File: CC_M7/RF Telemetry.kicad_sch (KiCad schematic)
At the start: 24 parts, among them U6 nRF52820-QDxx, U7 NRF21540-QDAA-R7, Y2 32MHz

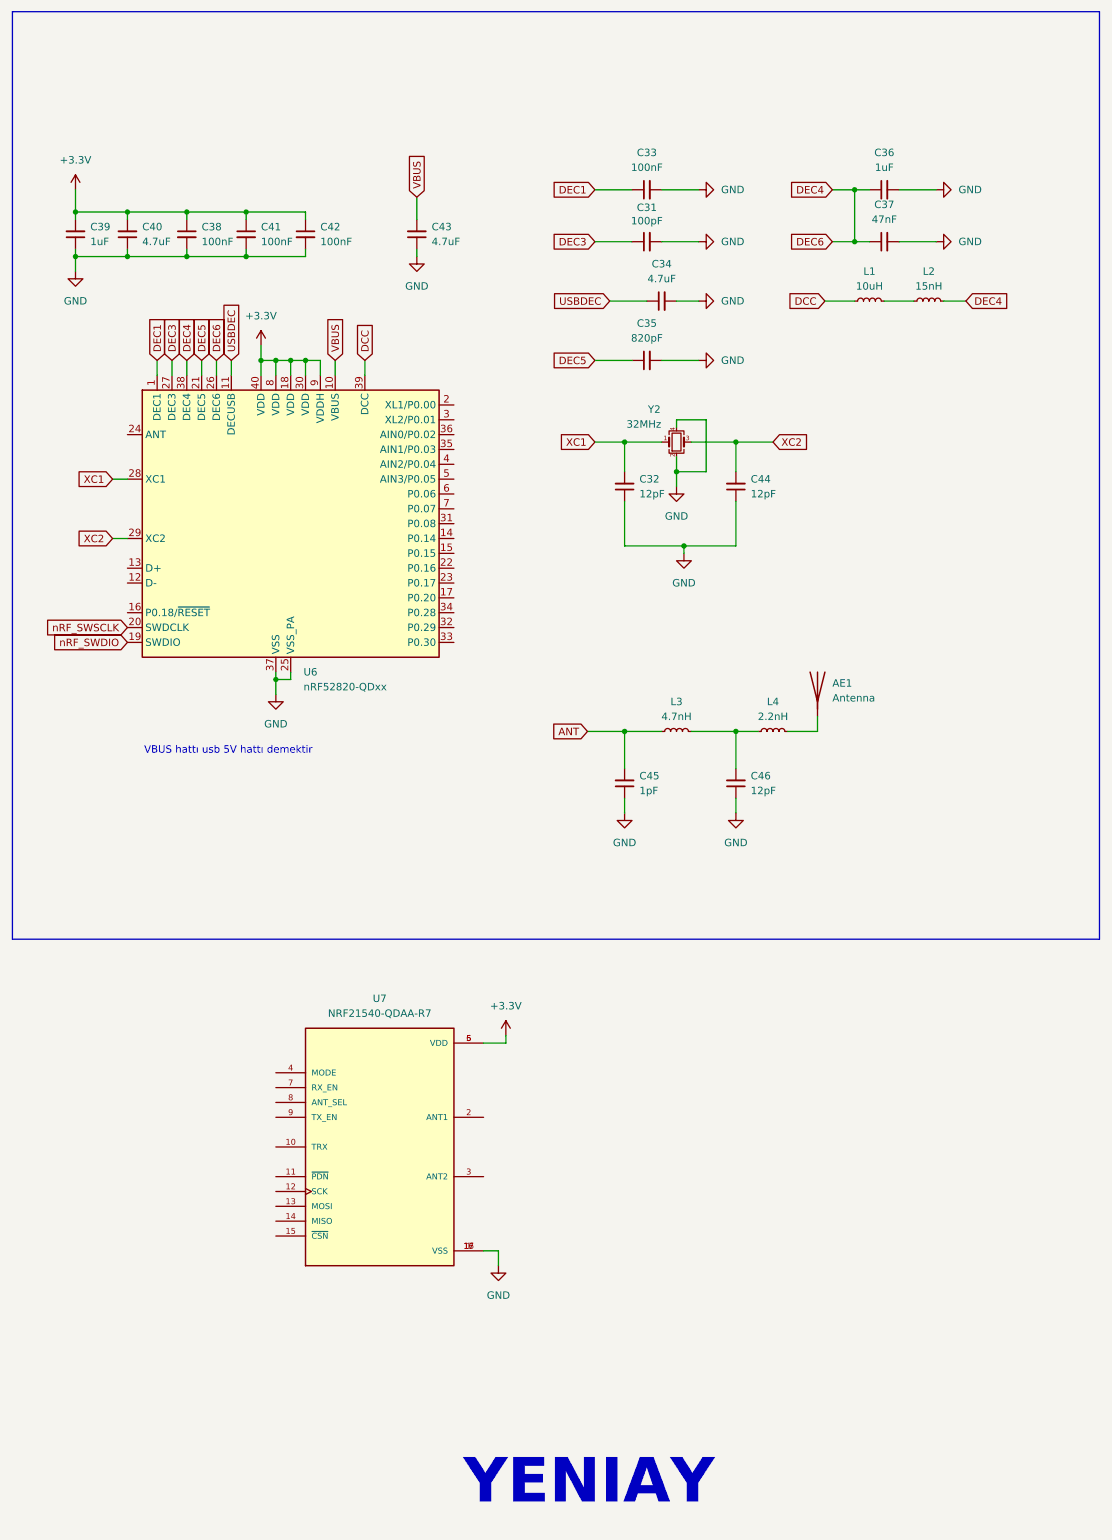
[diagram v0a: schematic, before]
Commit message: update
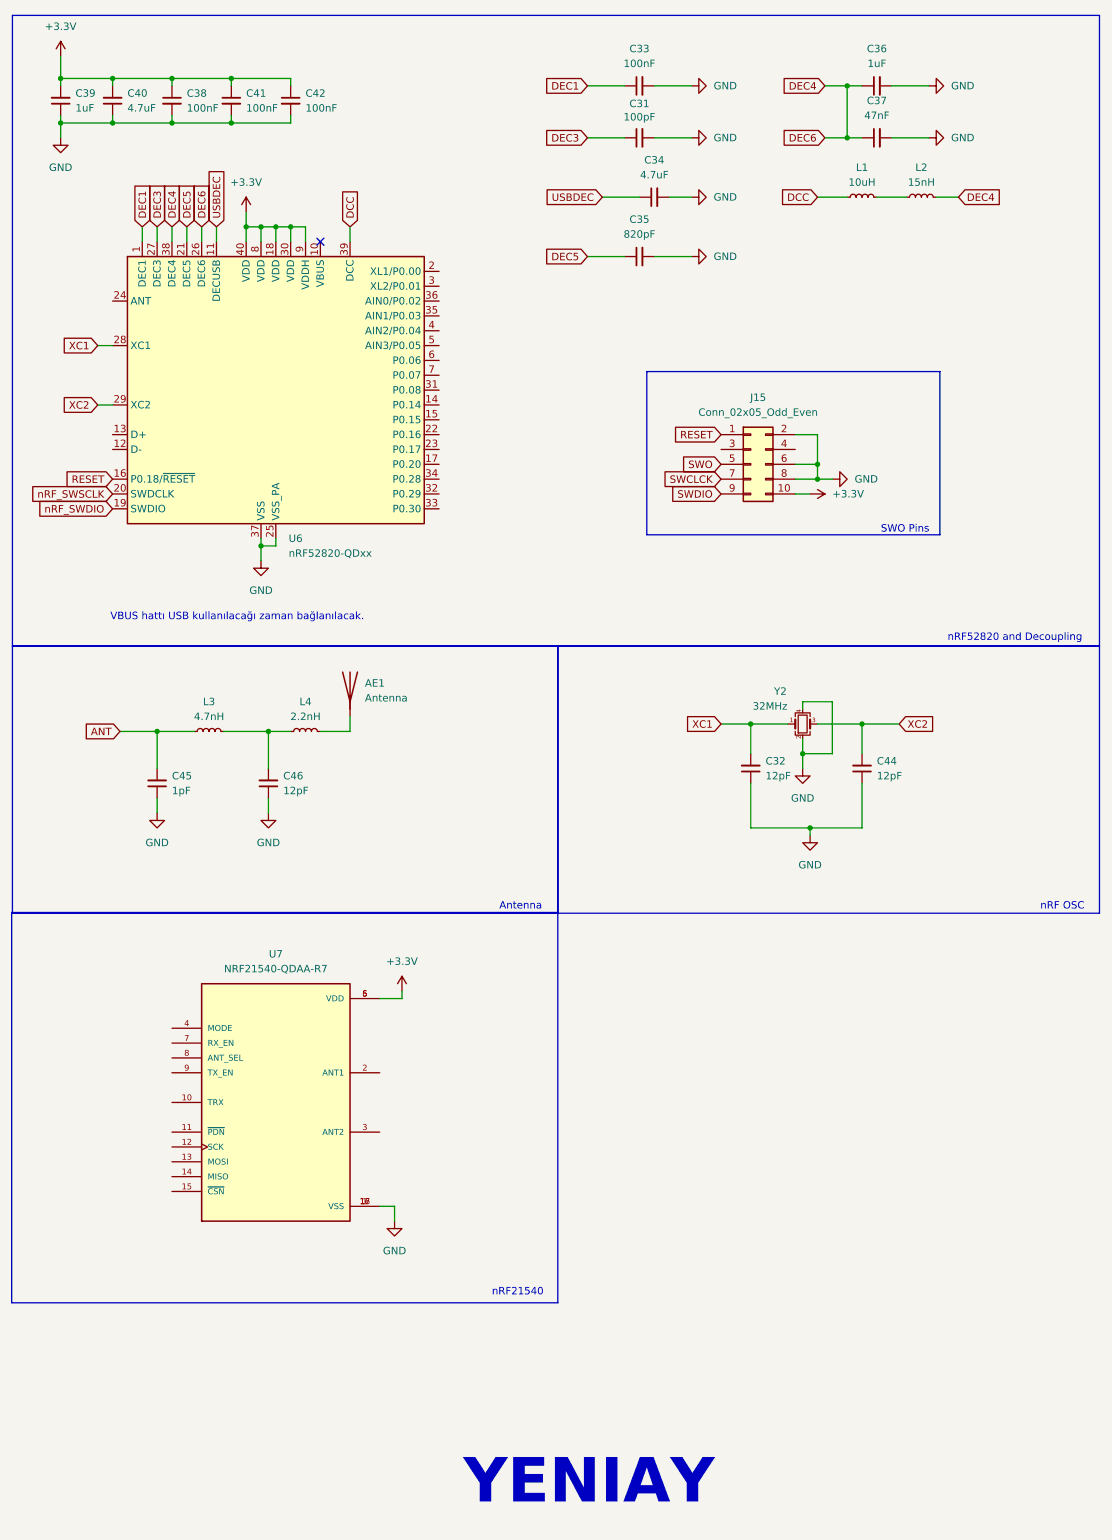
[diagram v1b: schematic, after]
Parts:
- removed C43: 4.7uF, symbol Device:C_Small
- added J15: Conn_02x05_Odd_Even, symbol Connector_Generic:Conn_02x05_Odd_Even
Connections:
- net +3.3V: now also J15.10 (Pin_10)
- net GND: now also J15.2 (Pin_2), J15.6 (Pin_6), J15.8 (Pin_8)
- net RESET: now reaches U6.16 (P0.18/~{RESET})
- net RESET: now also J15.1 (Pin_1)
- net VBUS: no longer names the net of U6.10 (VBUS)
- new net SWCLCK: J15.7 (Pin_7)
- new net SWDIO: J15.9 (Pin_9)
- new net SWO: J15.5 (Pin_5)
- no-connect marks 0 -> 1
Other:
- note added: "Antenna"
- note added: "SWO Pins"
- note added: "VBUS hattı USB kullanılacağı zaman bağlanılacak."
- note added: "nRF OSC"
- note added: "nRF21540"
- note added: "nRF52820 and Decoupling"
- note removed: "VBUS hattı usb 5V hattı demektir"
- moved on the sheet: AE1, C31, C32, C33, C34, C35, C36, C37, C38, C39, C40, C41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
